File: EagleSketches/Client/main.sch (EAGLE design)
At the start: 22 parts, among them J1 MICRO-SD-PUSH-PUSH-EXT-PIN, U1 LM386N

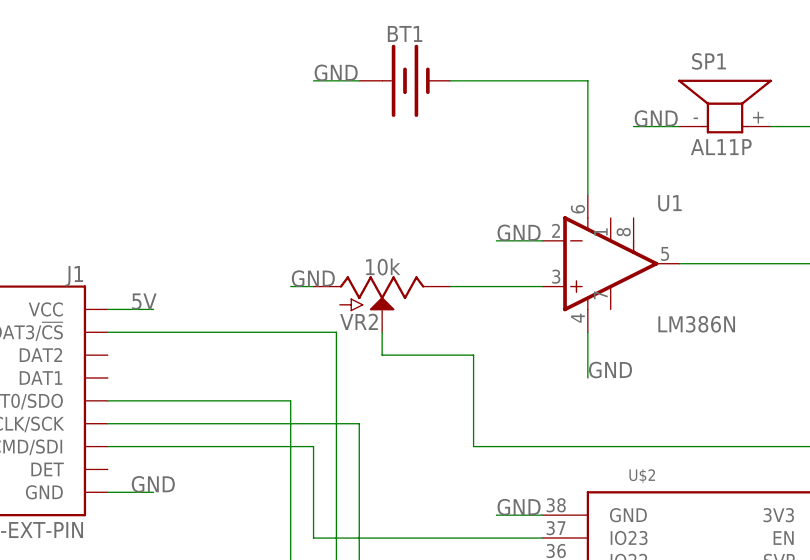
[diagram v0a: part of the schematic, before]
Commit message: Working audio
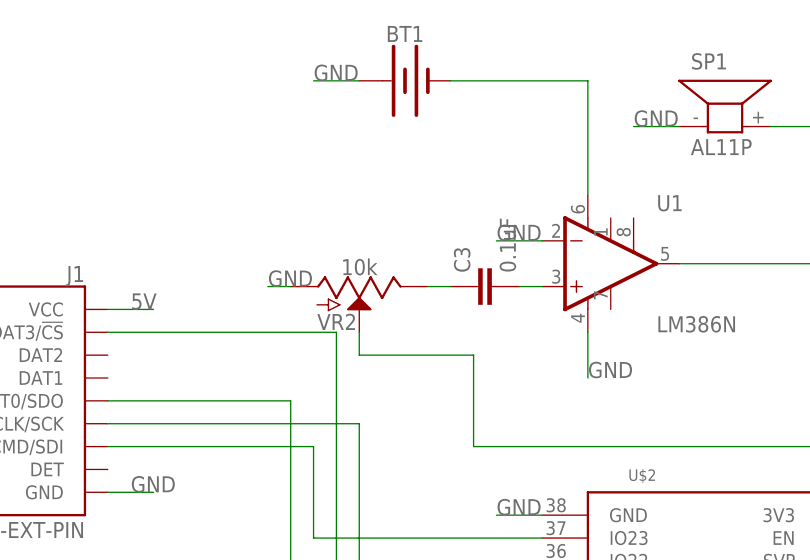
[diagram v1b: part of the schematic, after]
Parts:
- added C3: 0.1uF, SparkFun-Capacitors:0.1UF-KIT-EZ-50V-20%
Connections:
- new net N$30: C3.2, U1.+IN
- net N$23: now also C3.1; no longer U1.+IN
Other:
- moved on the sheet: VR2
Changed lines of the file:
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@@
 <part name="BT1" library="SparkFun-Batteries" deviceset="BATTERY" device="-9V"/>
 <part name="J1" library="SparkFun-Connectors" deviceset="MICRO-SD" device="-PUSH-PUSH-EXT-PIN"/>
+<part name="C3" library="SparkFun-Capacitors" deviceset="0.1UF" device="-KIT-EZ-50V-20%" value="0.1uF"/>
 </parts>
 <sheets>
@@
 <attribute name="VALUE" x="-15.24" y="106.68" size="1.778" layer="95" font="vector"/>
 </instance>
-<instance part="VR2" gate="G$1" x="-45.72" y="111.76" smashed="yes" rot="R270">
-<attribute name="NAME" x="-45.974" y="108.712" size="1.778" layer="95" font="vector" rot="R180"/>
-<attribute name="VALUE" x="-45.72" y="113.03" size="1.778" layer="95" font="vector" align="bottom-center"/>
+<instance part="VR2" gate="G$1" x="-48.26" y="111.76" smashed="yes" rot="R270">
+<attribute name="NAME" x="-48.514" y="108.712" size="1.778" layer="95" font="vector" rot="R180"/>
+<attribute name="VALUE" x="-48.26" y="113.03" size="1.778" layer="95" font="vector" align="bottom-center"/>
 </instance>
 <instance part="BT1" gate="G$1" x="-43.18" y="134.62" smashed="yes">
@@
 <attribute name="NAME" x="-78.74" y="112.268" size="1.778" layer="95" rot="MR0"/>
 <attribute name="VALUE" x="-78.74" y="83.82" size="1.778" layer="96" rot="MR0"/>
+</instance>
+<instance part="C3" gate="G$1" x="-33.02" y="111.76" smashed="yes" rot="R90">
+<attribute name="NAME" x="-35.941" y="113.284" size="1.778" layer="95" font="vector" rot="R90"/>
+<attribute name="VALUE" x="-30.861" y="113.284" size="1.778" layer="96" font="vector" rot="R90"/>
 </instance>
 </instances>
@@
 <segment>
 <pinref part="VR2" gate="G$1" pin="A"/>
-<wire x1="-53.34" y1="111.76" x2="-55.88" y2="111.76" width="0.1524" layer="91"/>
-<label x="-55.88" y="111.76" size="1.778" layer="95"/>
+<wire x1="-55.88" y1="111.76" x2="-58.42" y2="111.76" width="0.1524" layer="91"/>
+<label x="-58.42" y="111.76" size="1.778" layer="95"/>
 </segment>
 <segment>
@@
 </segment>
 </net>
-<net name="N$23" class="0">
-<segment>
-<pinref part="VR2" gate="G$1" pin="E"/>
-<pinref part="U1" gate="G1" pin="+IN"/>
-<wire x1="-38.1" y1="111.76" x2="-27.94" y2="111.76" width="0.1524" layer="91"/>
-</segment>
-</net>
 <net name="N$21" class="0">
 <segment>
 <pinref part="VR2" gate="G$1" pin="S"/>
 <wire x1="-35.56" y1="93.98" x2="-35.56" y2="104.14" width="0.1524" layer="91"/>
-<wire x1="-35.56" y1="104.14" x2="-45.72" y2="104.14" width="0.1524" layer="91"/>
-<wire x1="-45.72" y1="104.14" x2="-45.72" y2="106.68" width="0.1524" layer="91"/>
+<wire x1="-35.56" y1="104.14" x2="-48.26" y2="104.14" width="0.1524" layer="91"/>
+<wire x1="-48.26" y1="104.14" x2="-48.26" y2="106.68" width="0.1524" layer="91"/>
 <pinref part="U$2" gate="G$1" pin="IO25"/>
 <wire x1="7.62" y1="66.04" x2="10.16" y2="66.04" width="0.1524" layer="91"/>
@@
 </segment>
 </net>
+<net name="N$23" class="0">
+<segment>
+<pinref part="VR2" gate="G$1" pin="E"/>
+<pinref part="C3" gate="G$1" pin="1"/>
+<wire x1="-40.64" y1="111.76" x2="-38.1" y2="111.76" width="0.1524" layer="91"/>
+</segment>
+</net>
+<net name="N$30" class="0">
+<segment>
+<pinref part="C3" gate="G$1" pin="2"/>
+<pinref part="U1" gate="G1" pin="+IN"/>
+<wire x1="-30.48" y1="111.76" x2="-27.94" y2="111.76" width="0.1524" layer="91"/>
+</segment>
+</net>
